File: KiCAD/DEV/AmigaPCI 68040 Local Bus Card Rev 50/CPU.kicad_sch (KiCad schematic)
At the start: 22 parts, among them J100 SNOOP, U200 MC68040, U203 74LVC245

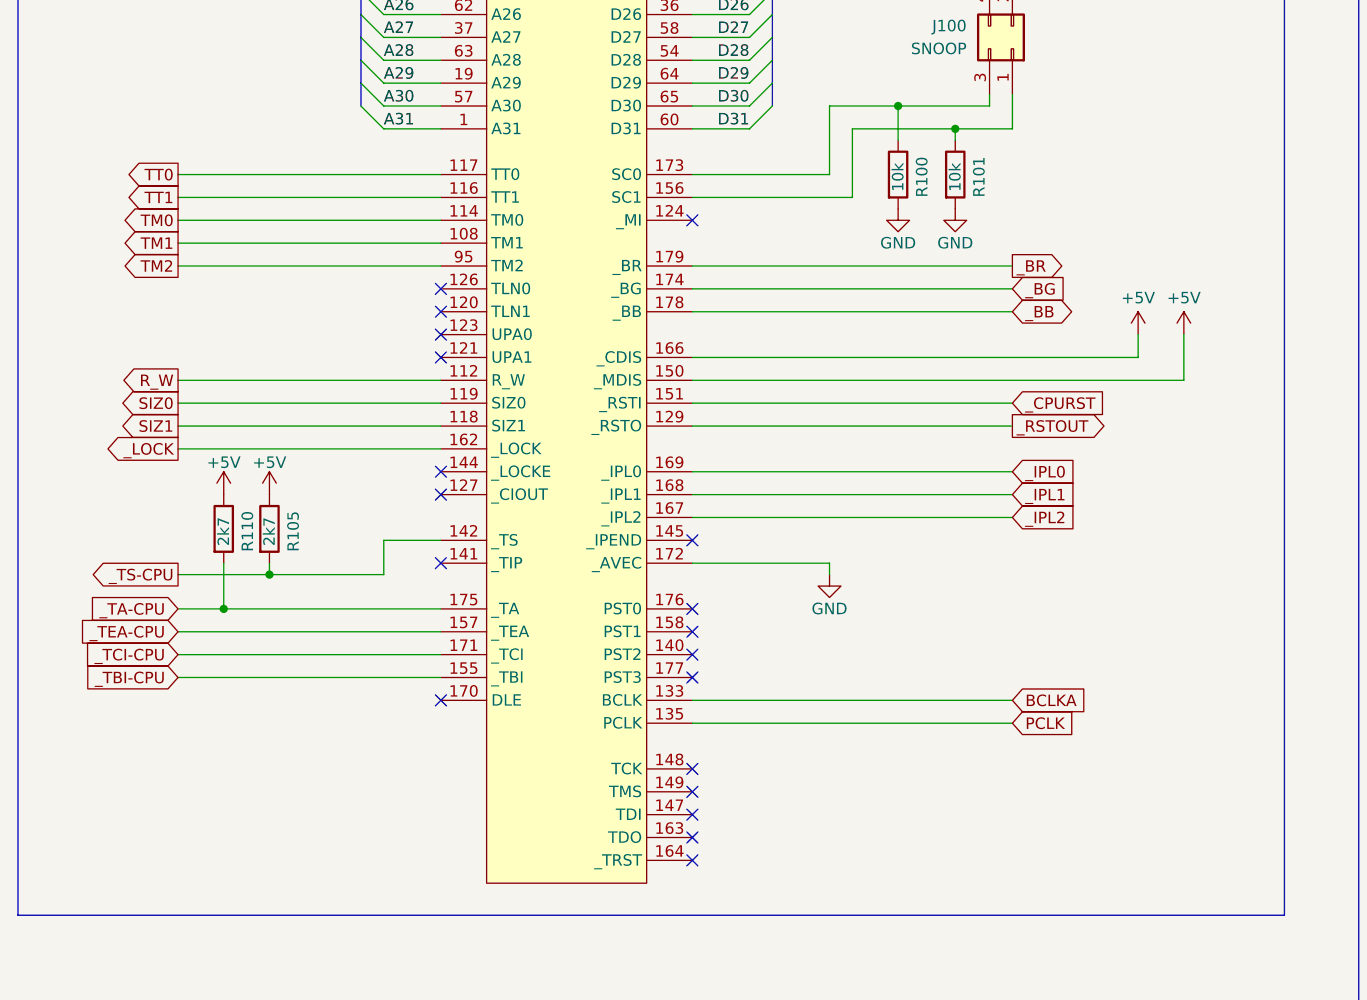
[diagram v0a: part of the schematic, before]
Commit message: CPU Card Rev 5.0 - Connect _MI to U400.
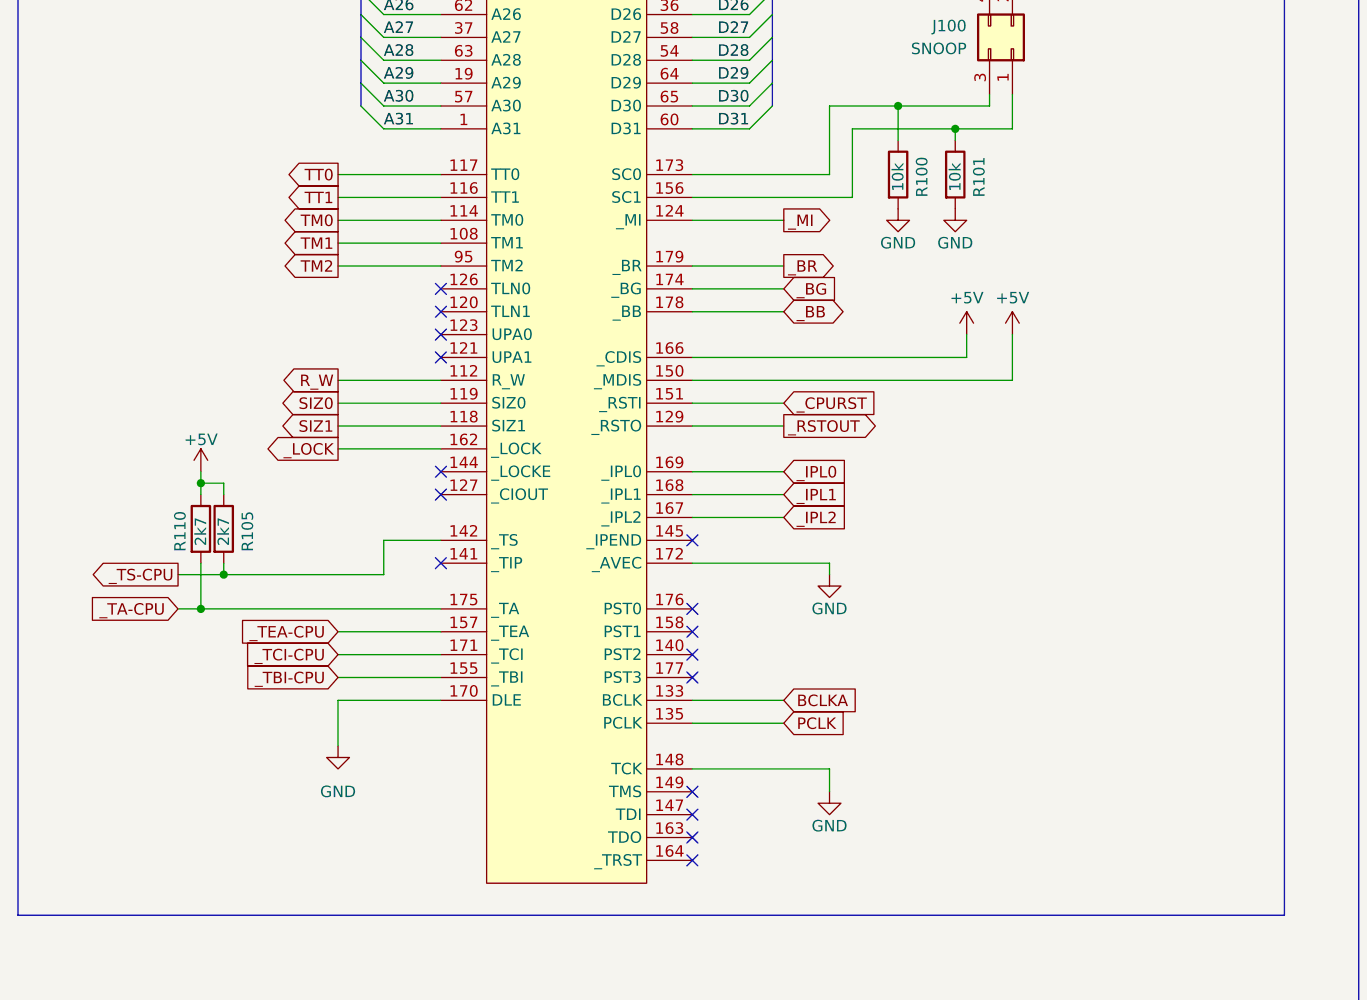
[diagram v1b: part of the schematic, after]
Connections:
- net GND: now also U200.148 (TCK), U200.170 (DLE)
- net _MI: now reaches U200.124 (_MI)
- no-connect marks 23 -> 20
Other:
- moved on the sheet: R105, R110
